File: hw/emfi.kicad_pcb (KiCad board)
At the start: 2 copper layers, 132.5 x 38 mm, 81 parts, among them J1 USB_B_Micro, J2 Conn_Coaxial, J3 Conn_Coaxial, J4 Conn_01x02, J5 Conn_01x03, J6 Conn_Coaxial, Q1 STT6N3LLH6, Q2 IKW40N120H3FKSA1, U1 STM32F205RETx, U2 FT232RL, U3 MIC2288, U4 LD1117S33TR_SOT223, U5 LD1117S33TR_SOT223, U6 MCP1407-E/SN, U7 SCS-200LD, U8 74LVC1G32

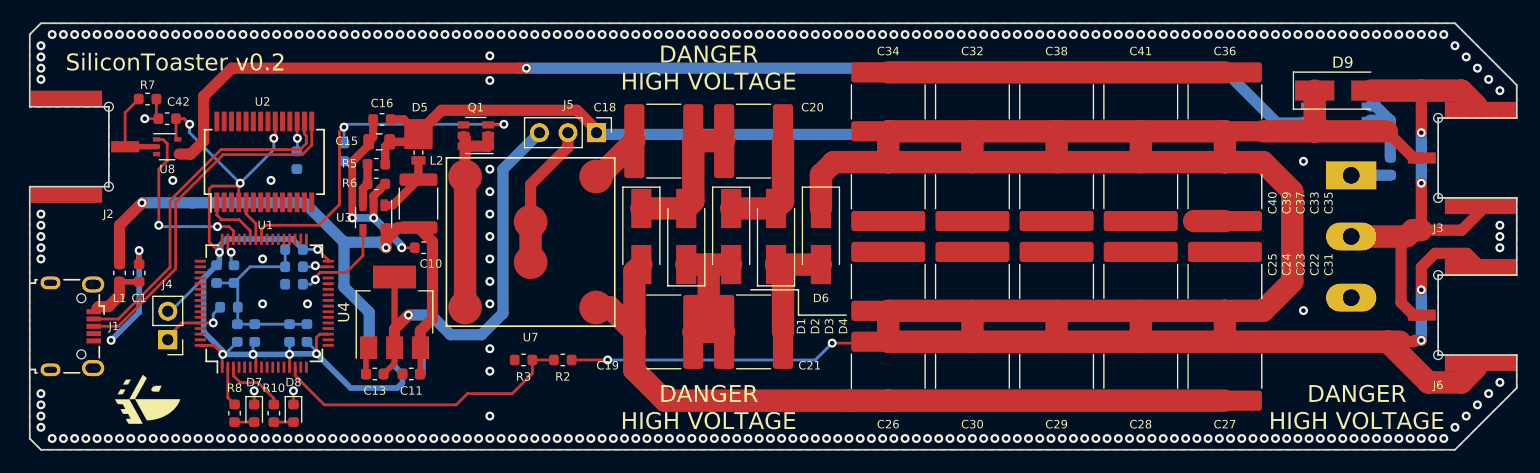
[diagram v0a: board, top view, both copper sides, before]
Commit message: Updates to silicon-toaster for components you can buy
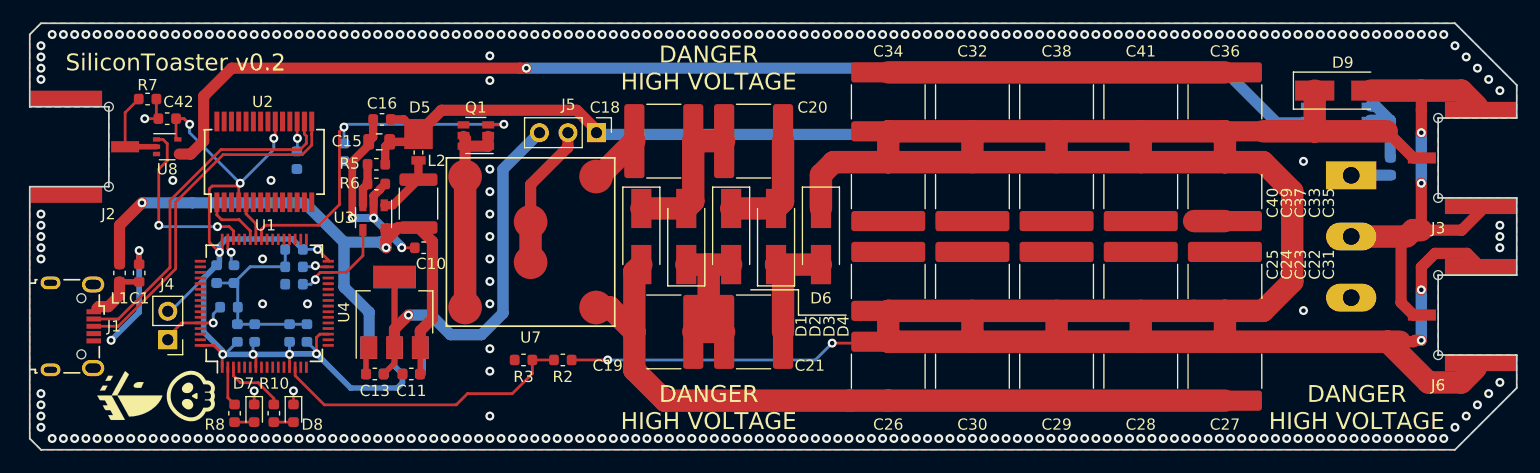
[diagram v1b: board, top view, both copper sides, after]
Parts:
- added G***: LOGO, Skull:skull_logo, F.Cu at (57.4, 61.2)
- moved LOGO1 1.62 mm to (51.9, 61.2)
